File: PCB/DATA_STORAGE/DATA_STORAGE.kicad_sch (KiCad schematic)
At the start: 12 parts, among them IC1 CY15B108QN-40SXI, J1 Conn_02x06_Odd_Even, J2 Conn_02x06_Odd_Even, J3 1660, Q1 DMG2305UX-7, Q2 PJE8408_R1_00001

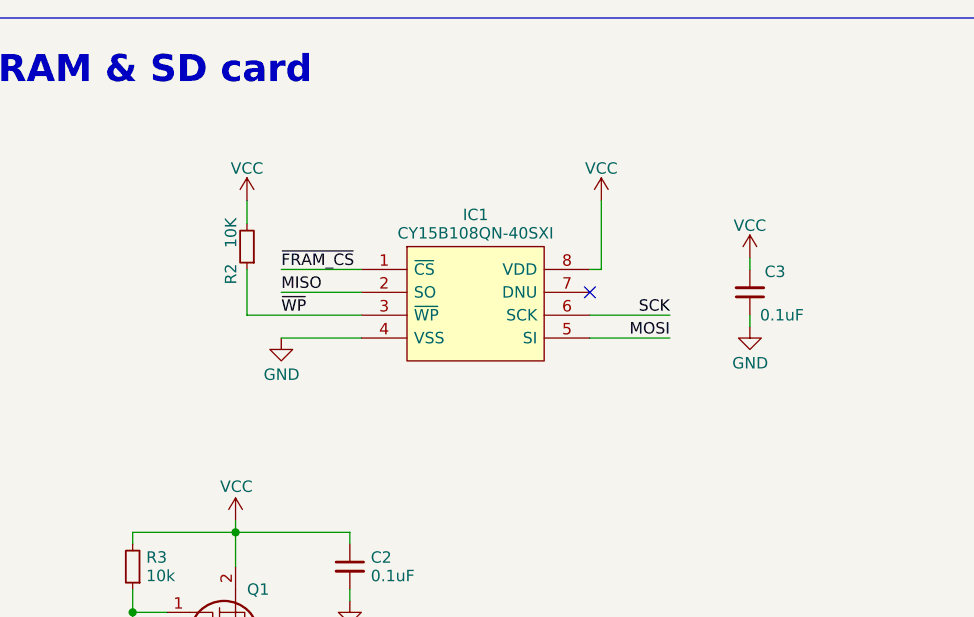
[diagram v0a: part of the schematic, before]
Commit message: udated by FZ from Windows
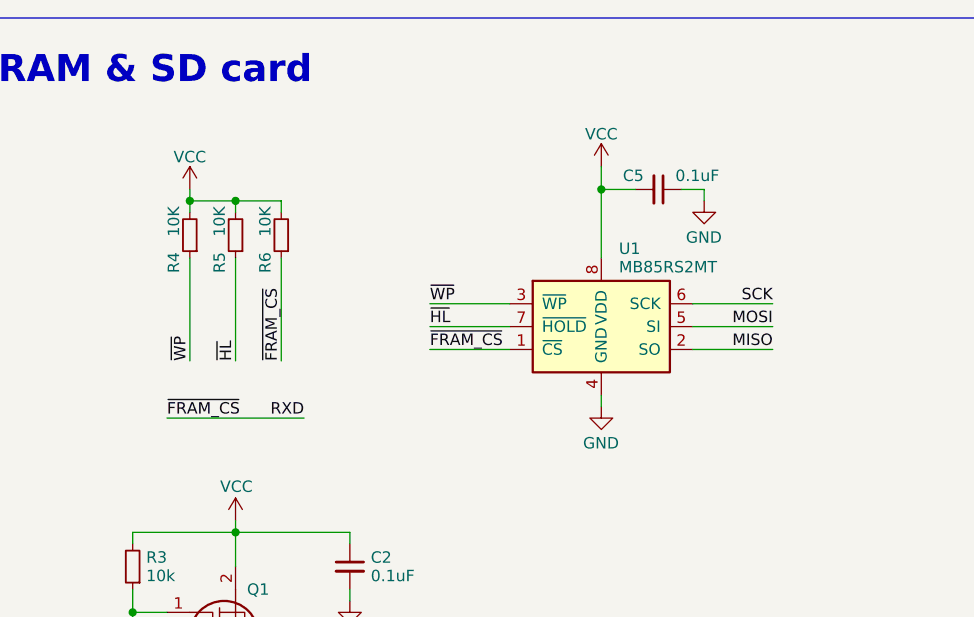
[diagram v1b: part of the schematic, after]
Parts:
- removed C3: 0.1uF, Capacitor_SMD:C_0603_1608Metric_Pad1.08x0.95mm_HandSolder, symbol Device:C_Small
- removed IC1: CY15B108QN-40SXI, SamacSys_Parts:SOIC127P800X203-8N, symbol SamacSys_Parts:CY15B108QN-40SXI
- removed R2: 10K, Resistor_SMD:R_0402_1005Metric_Pad0.72x0.64mm_HandSolder, symbol Device:R_Small
- added C5: 0.1uF, Capacitor_SMD:C_0603_1608Metric_Pad1.08x0.95mm_HandSolder, symbol Device:C_Small
- added R4, R5, R6: 10K, Resistor_SMD:R_0603_1608Metric_Pad0.98x0.95mm_HandSolder, symbol Device:R_Small
- added U1: MB85RS2MT, Package_SO:SSOP-8_3.9x5.05mm_P1.27mm, symbol Memory_NVRAM:MB85RS2MT
- Q2: footprint SOTFL50P160X60-3N -> SamacSys_Parts:SOTFL50P160X60-3N
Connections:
- net GND: now also C5.1, U1.4 (GND)
- net MISO: now also U1.2 (SO)
- net MOSI: now also U1.5 (SI)
- net RXD: now also R6.1, U1.1 (~{CS})
- net SCK: now also U1.6 (SCK)
- net VCC: now also C5.2, R4.2, R5.2, R6.2, U1.8 (VDD)
- net ~{WP}: now also R4.1, U1.3 (~{WP})
- new net ~{HL}: R5.1, U1.7 (~{HOLD})
- no-connect marks 4 -> 3
